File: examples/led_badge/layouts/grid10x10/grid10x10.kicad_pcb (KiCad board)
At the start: 4 copper layers, 200 parts

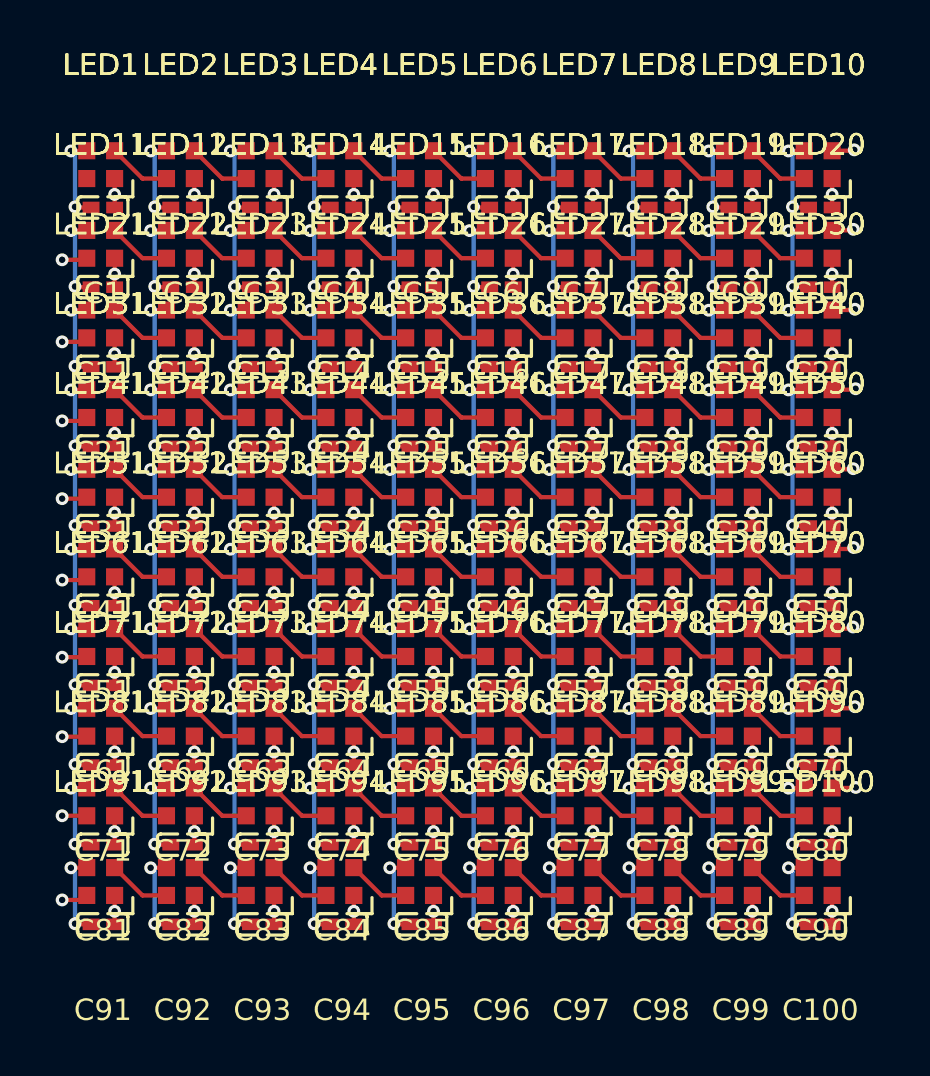
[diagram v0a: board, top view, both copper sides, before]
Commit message: rebuild lad badge
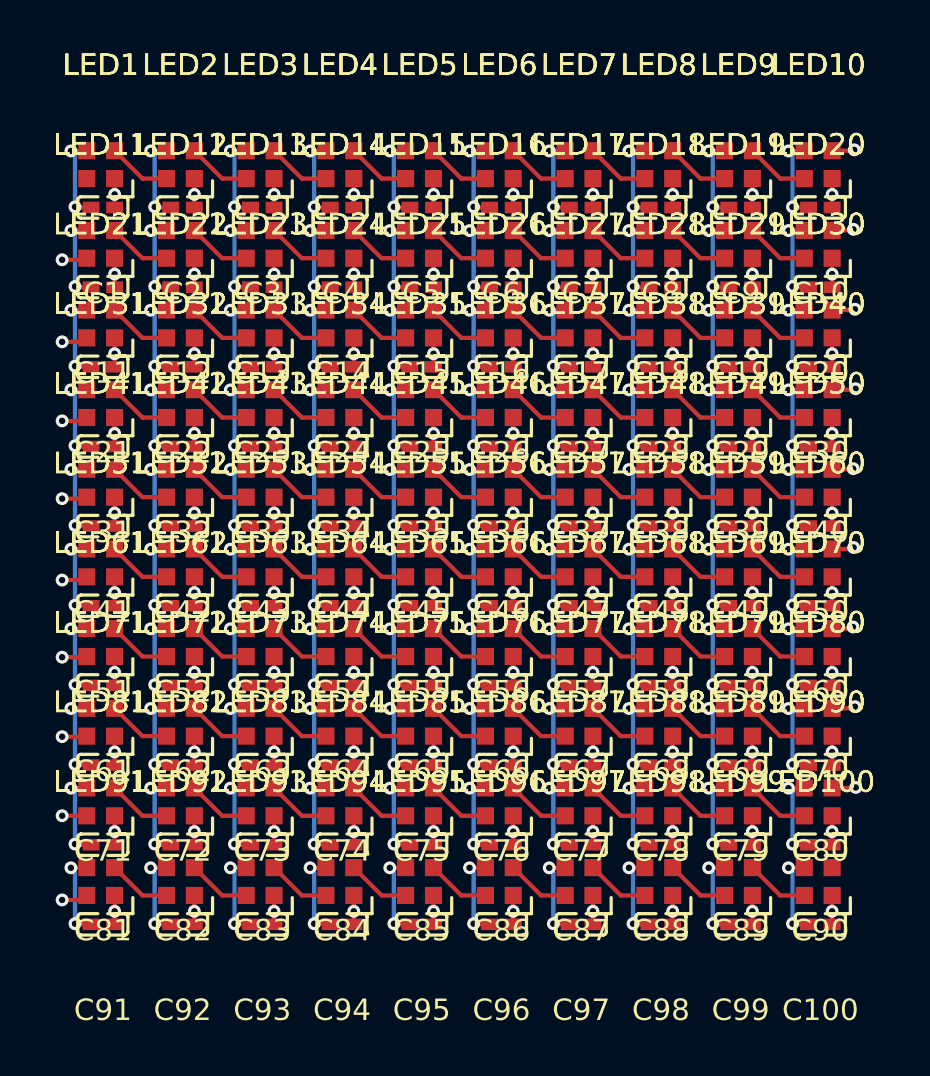
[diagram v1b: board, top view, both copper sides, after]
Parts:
- C1, C10, C100, C11, C12, C13, C14, C15, C16, C17, C18, C19, C2, C20, C21, C22, C23, C24, C25, C26, C27, C28, C29, C3, C30, C31, C32, C33, C34, C35, C36, C37, C38, C39, C4, C40, C41, C42, C43, C44, C45, C46, C47, C48, C49, C5, C50, C51, C52, C53, C54, C55, C56, C57, C58, C59, C6, C60, C61, C62, C63, C64, C65, C66, C67, C68, C69, C7, C70, C71, C72, C73, C74, C75, C76, C77, C78, C79, C8, C80, C81, C82, C83, C84, C85, C86, C87, C88, C89, C9, C90, C91, C92, C93, C94, C95, C96, C97, C98, C99: value 100nF ±10% 16V X7R -> 100nF ±10% 50V X7R; footprint Samsung_Electro_Mechanics_CL05B104KO5NNNC:C0402 -> Samsung_Electro_Mechanics_CL05B104KB54PNC:C0402
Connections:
- net -line-0 renamed rows[0]-data_in-line
- net -line-1 renamed data_out-line
- net -line-10 renamed rows[9]-data_in-line
- net -line-2 renamed rows[1]-data_in-line
- net -line-3 renamed rows[2]-data_in-line
- net -line-4 renamed rows[3]-data_in-line
- net -line-5 renamed rows[4]-data_in-line
- net -line-6 renamed rows[5]-data_in-line
- net -line-7 renamed rows[6]-data_in-line
- net -line-8 renamed rows[7]-data_in-line
- net -line-9 renamed rows[8]-data_in-line
- net gnd renamed GND
- net hv renamed VCC
- net rows[0]-DOUT-0 renamed leds[1]-data_in-DIN-0
- net rows[0]-DOUT-1 renamed leds[2]-data_in-DIN-0
- net rows[0]-DOUT-2 renamed leds[3]-data_in-DIN-0
- net rows[0]-DOUT-3 renamed leds[4]-data_in-DIN-0
- net rows[0]-DOUT-4 renamed leds[5]-data_in-DIN-0
- net rows[0]-DOUT-5 renamed leds[6]-data_in-DIN-0
- net rows[0]-DOUT-6 renamed leds[7]-data_in-DIN-0
- net rows[0]-DOUT-7 renamed leds[8]-data_in-DIN-0
- net rows[0]-DOUT-8 renamed leds[9]-data_in-DIN-0
- net rows[1]-DOUT-0 renamed leds[1]-data_in-DIN-1
- net rows[1]-DOUT-1 renamed leds[2]-data_in-DIN-1
- net rows[1]-DOUT-2 renamed leds[3]-data_in-DIN-1
- net rows[1]-DOUT-3 renamed leds[4]-data_in-DIN-1
- net rows[1]-DOUT-4 renamed leds[5]-data_in-DIN-1
- net rows[1]-DOUT-5 renamed leds[6]-data_in-DIN-1
- net rows[1]-DOUT-6 renamed leds[7]-data_in-DIN-1
- net rows[1]-DOUT-7 renamed leds[8]-data_in-DIN-1
- net rows[1]-DOUT-8 renamed leds[9]-data_in-DIN-1
- net rows[2]-DOUT-0 renamed leds[1]-data_in-DIN-2
- net rows[2]-DOUT-1 renamed leds[2]-data_in-DIN-2
- net rows[2]-DOUT-2 renamed leds[3]-data_in-DIN-2
- net rows[2]-DOUT-3 renamed leds[4]-data_in-DIN-2
- net rows[2]-DOUT-4 renamed leds[5]-data_in-DIN-2
- net rows[2]-DOUT-5 renamed leds[6]-data_in-DIN-2
- net rows[2]-DOUT-6 renamed leds[7]-data_in-DIN-2
- net rows[2]-DOUT-7 renamed leds[8]-data_in-DIN-2
- net rows[2]-DOUT-8 renamed leds[9]-data_in-DIN-2
- net rows[3]-DOUT-0 renamed leds[1]-data_in-DIN-3
- net rows[3]-DOUT-1 renamed leds[2]-data_in-DIN-3
- net rows[3]-DOUT-2 renamed leds[3]-data_in-DIN-3
- net rows[3]-DOUT-3 renamed leds[4]-data_in-DIN-3
- net rows[3]-DOUT-4 renamed leds[5]-data_in-DIN-3
- net rows[3]-DOUT-5 renamed leds[6]-data_in-DIN-3
- net rows[3]-DOUT-6 renamed leds[7]-data_in-DIN-3
- net rows[3]-DOUT-7 renamed leds[8]-data_in-DIN-3
- net rows[3]-DOUT-8 renamed leds[9]-data_in-DIN-3
- net rows[4]-DOUT-0 renamed leds[1]-data_in-DIN-4
- net rows[4]-DOUT-1 renamed leds[2]-data_in-DIN-4
- net rows[4]-DOUT-2 renamed leds[3]-data_in-DIN-4
- net rows[4]-DOUT-3 renamed leds[4]-data_in-DIN-4
- net rows[4]-DOUT-4 renamed leds[5]-data_in-DIN-4
- net rows[4]-DOUT-5 renamed leds[6]-data_in-DIN-4
- net rows[4]-DOUT-6 renamed leds[7]-data_in-DIN-4
- net rows[4]-DOUT-7 renamed leds[8]-data_in-DIN-4
- net rows[4]-DOUT-8 renamed leds[9]-data_in-DIN-4
- net rows[5]-DOUT-0 renamed leds[1]-data_in-DIN-5
- net rows[5]-DOUT-1 renamed leds[2]-data_in-DIN-5
- net rows[5]-DOUT-2 renamed leds[3]-data_in-DIN-5
- net rows[5]-DOUT-3 renamed leds[4]-data_in-DIN-5
- net rows[5]-DOUT-4 renamed leds[5]-data_in-DIN-5
- net rows[5]-DOUT-5 renamed leds[6]-data_in-DIN-5
- net rows[5]-DOUT-6 renamed leds[7]-data_in-DIN-5
- net rows[5]-DOUT-7 renamed leds[8]-data_in-DIN-5
- net rows[5]-DOUT-8 renamed leds[9]-data_in-DIN-5
- net rows[6]-DOUT-0 renamed leds[1]-data_in-DIN-6
- net rows[6]-DOUT-1 renamed leds[2]-data_in-DIN-6
- net rows[6]-DOUT-2 renamed leds[3]-data_in-DIN-6
- net rows[6]-DOUT-3 renamed leds[4]-data_in-DIN-6
- net rows[6]-DOUT-4 renamed leds[5]-data_in-DIN-6
- net rows[6]-DOUT-5 renamed leds[6]-data_in-DIN-6
- net rows[6]-DOUT-6 renamed leds[7]-data_in-DIN-6
- net rows[6]-DOUT-7 renamed leds[8]-data_in-DIN-6
- net rows[6]-DOUT-8 renamed leds[9]-data_in-DIN-6
- net rows[7]-DOUT-0 renamed leds[1]-data_in-DIN-7
- net rows[7]-DOUT-1 renamed leds[2]-data_in-DIN-7
- net rows[7]-DOUT-2 renamed leds[3]-data_in-DIN-7
- net rows[7]-DOUT-3 renamed leds[4]-data_in-DIN-7
- net rows[7]-DOUT-4 renamed leds[5]-data_in-DIN-7
- net rows[7]-DOUT-5 renamed leds[6]-data_in-DIN-7
- net rows[7]-DOUT-6 renamed leds[7]-data_in-DIN-7
- net rows[7]-DOUT-7 renamed leds[8]-data_in-DIN-7
- net rows[7]-DOUT-8 renamed leds[9]-data_in-DIN-7
- net rows[8]-DOUT-0 renamed leds[1]-data_in-DIN-8
- net rows[8]-DOUT-1 renamed leds[2]-data_in-DIN-8
- net rows[8]-DOUT-2 renamed leds[3]-data_in-DIN-8
- net rows[8]-DOUT-3 renamed leds[4]-data_in-DIN-8
- net rows[8]-DOUT-4 renamed leds[5]-data_in-DIN-8
- net rows[8]-DOUT-5 renamed leds[6]-data_in-DIN-8
- net rows[8]-DOUT-6 renamed leds[7]-data_in-DIN-8
- net rows[8]-DOUT-7 renamed leds[8]-data_in-DIN-8
- net rows[8]-DOUT-8 renamed leds[9]-data_in-DIN-8
- net rows[9]-DOUT-0 renamed leds[1]-data_in-DIN-9
- net rows[9]-DOUT-1 renamed leds[2]-data_in-DIN-9
- net rows[9]-DOUT-2 renamed leds[3]-data_in-DIN-9
- net rows[9]-DOUT-3 renamed leds[4]-data_in-DIN-9
- net rows[9]-DOUT-4 renamed leds[5]-data_in-DIN-9
- net rows[9]-DOUT-5 renamed leds[6]-data_in-DIN-9
- net rows[9]-DOUT-6 renamed leds[7]-data_in-DIN-9
- net rows[9]-DOUT-7 renamed leds[8]-data_in-DIN-9
- net rows[9]-DOUT-8 renamed leds[9]-data_in-DIN-9
